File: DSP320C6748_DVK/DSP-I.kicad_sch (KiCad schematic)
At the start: 35 parts, among them J1 USB_A, J2 JTAG, U1 TMS320C6748EZWT4, Y1 ASE-24.000MHZ-LC-T, Y2 FX135A-327

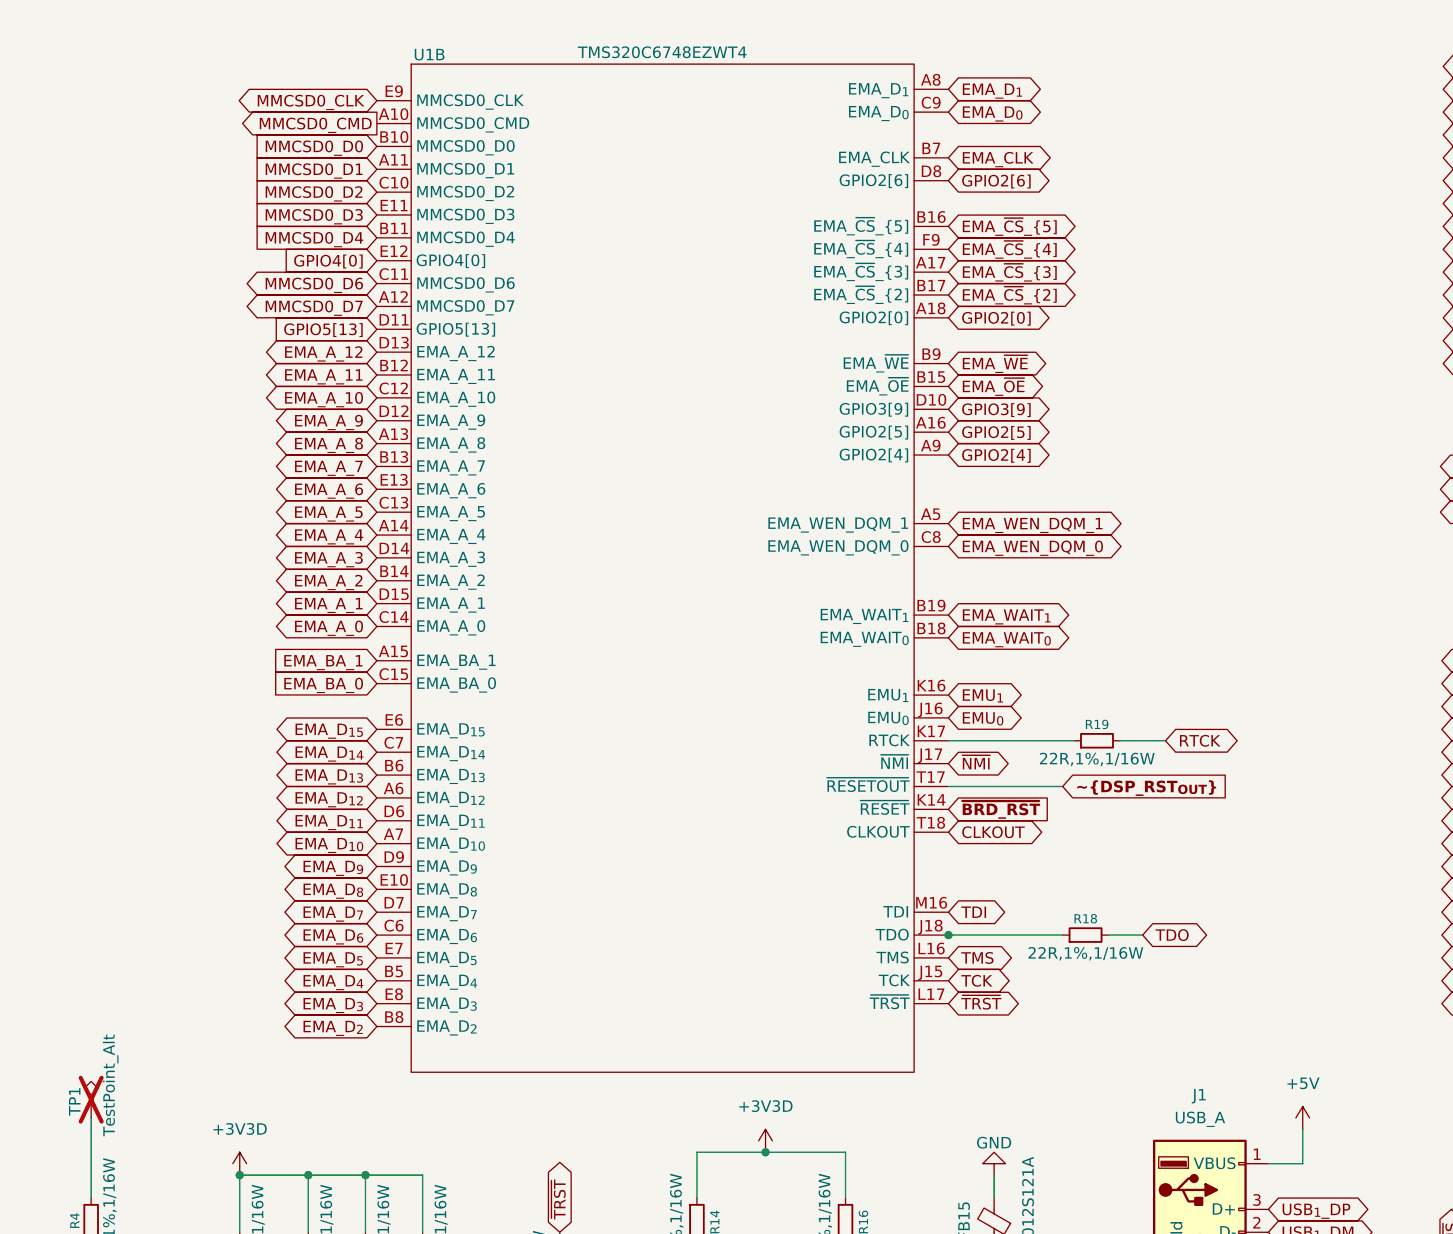
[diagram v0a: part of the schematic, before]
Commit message: Schematic Corrections-II Done
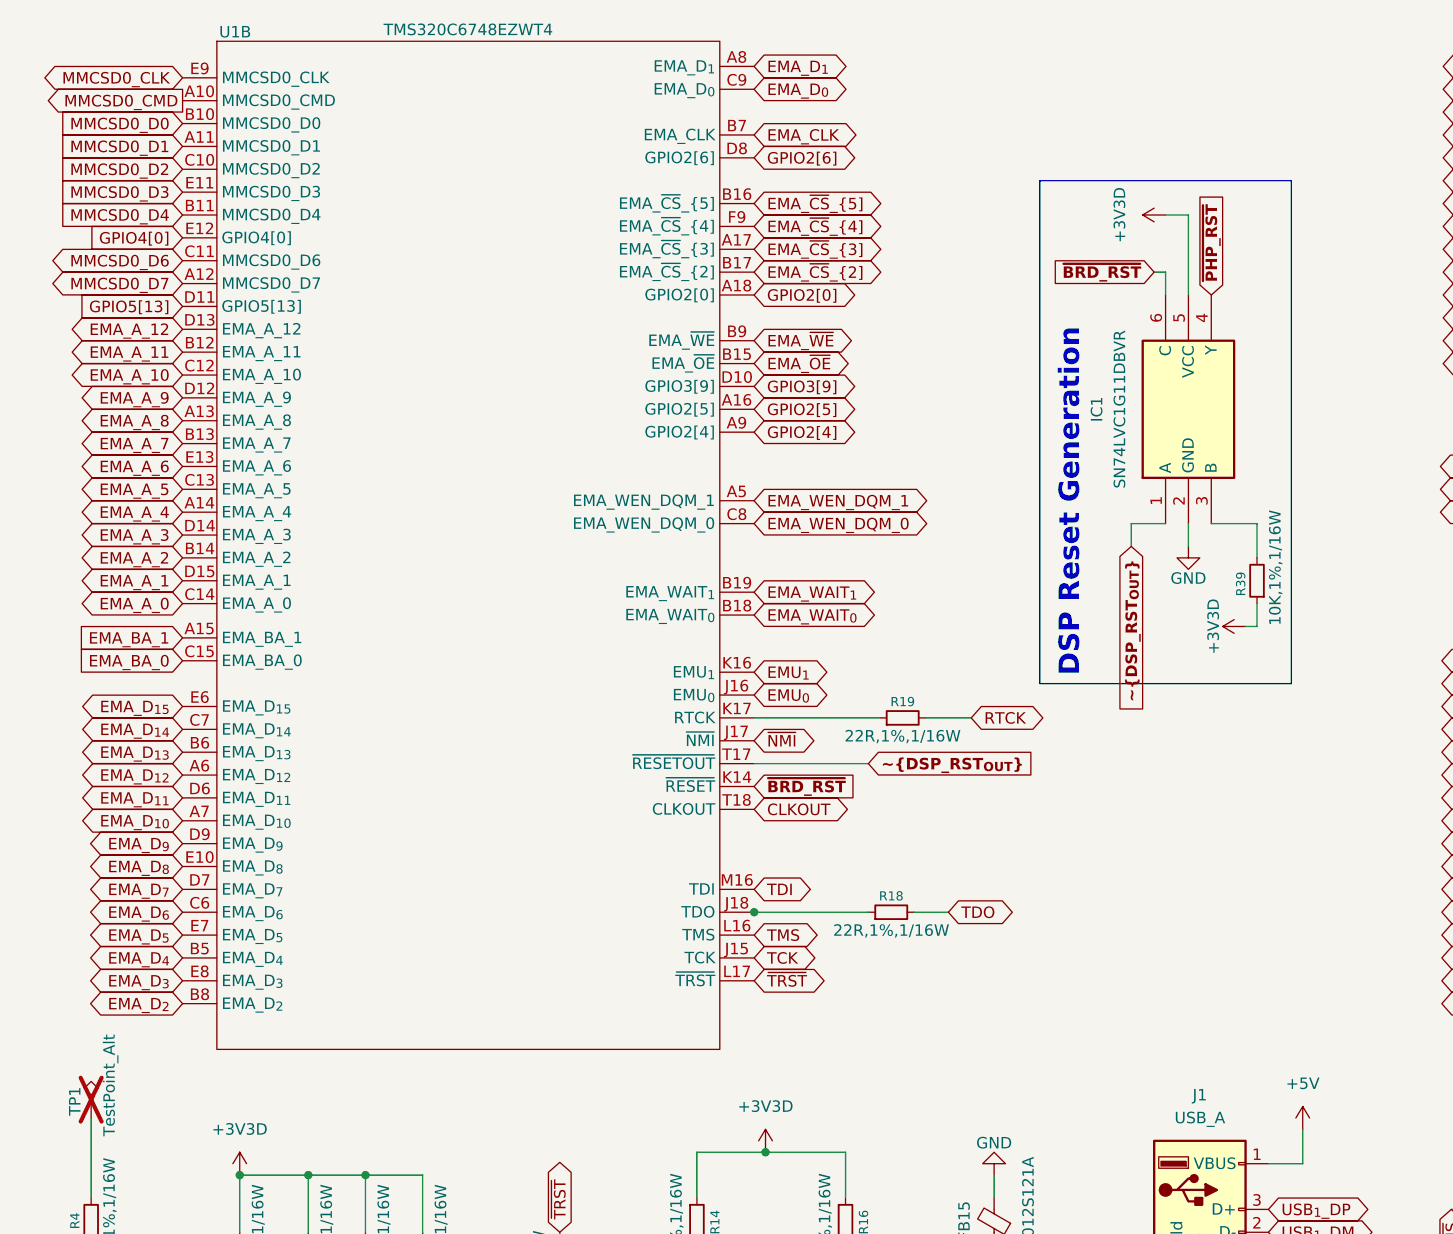
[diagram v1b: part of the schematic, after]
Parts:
- added IC1: SN74LVC1G11DBVR, SOT95P280X145-6N, symbol SN74LVC1G11DBVR:SN74LVC1G11DBVR
- added R39: 10K,1%,1/16W, symbol Device:R_Small
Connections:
- net +3V3D: now also IC1.5 (VCC), R39.1
- net GND: now also IC1.2 (GND)
- net ~{BRD_RST}: now also IC1.6 (C)
- net ~{DSP_RST_{OUT}}: now also IC1.1 (A)
- new net: IC1.3 (B), R39.2
- new net ~{PHP_RST}: IC1.4 (Y)
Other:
- note added: "DSP Reset Generation"
- moved on the sheet: R18, R19, U1B
